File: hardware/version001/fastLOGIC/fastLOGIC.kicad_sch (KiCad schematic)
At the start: 82 parts, among them J1 AVR-ISP-6, J10 0-5V_ANALOG_IN_A, J11 PRES_SENS_BOTTOM, J12 PRES_SENS_TOP, J13 0-5V_ANALOG_IN_B, J14 RELAY_OUT_B, J15 RELAY_OUT_A, J2 USB_B_Micro, J3 DS18B20, J4 12-24V, J5 I2C, J8 12-24V_IN_A, J9 12-24V_IN_B, K1 SANYOU_SRD_Form_C, K2 SANYOU_SRD_Form_C, Q1 MMBT5551L, Q2 MMBT5551L, SW1 SET, SW2 reset, SW3 PLUS, SW4 MINUS, U1 LM78M05_TO252, U2 ATmega328P-A, U3 EL817, U4 EL817, U5 CP2102N-Axx-xQFN28, U6 TM1637, U7 CA56-12SRWA, Y1 Crystal_25MHz

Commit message: hardware chnages minor
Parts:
- removed J2: USB_B_Micro, Connector_USB:USB_Micro-B_Amphenol_10118194_Horizontal, symbol Connector:USB_B_Micro
- added J6: USB_B_Mini, Connector_USB:USB_Mini-B_Tensility_54-00023_Vertical, symbol Connector:USB_B_Mini
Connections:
- net GND: now also J6.5 (GND)
- net at C14.2, C15.2, U5.7 (VREGIN)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: now also J6.1 (VBUS)
- net at U5.5 (D-): now also J6.2 (D-)
- net at U5.4 (D+): now also J6.3 (D+)
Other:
- moved on the sheet: C1, C10, C11, C12, C13, C14, C15, C16, C17, C2, C3, C4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

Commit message: latest pcb
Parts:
- U3, U4: footprint Package_DIP:DIP-4_W7.62mm_SMDSocket_SmallPads -> Package_DIP:DIP-4_W8.89mm_SMDSocket_LongPads
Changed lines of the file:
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@@
       (effects (font (size 1.27 1.27)))
     )
-    (property "Footprint" "Package_DIP:DIP-4_W7.62mm_SMDSocket_SmallPads" (at 54.737 194.691 0)
+    (property "Footprint" "Package_DIP:DIP-4_W8.89mm_SMDSocket_LongPads" (at 54.737 194.691 0)
       (effects (font (size 1.27 1.27) italic) (justify left) hide)
     )
@@
       (effects (font (size 1.27 1.27)))
     )
-    (property "Footprint" "Package_DIP:DIP-4_W7.62mm_SMDSocket_SmallPads" (at 91.821 197.993 0)
+    (property "Footprint" "Package_DIP:DIP-4_W8.89mm_SMDSocket_LongPads" (at 91.821 197.993 0)
       (effects (font (size 1.27 1.27) italic) (justify left) hide)
     )

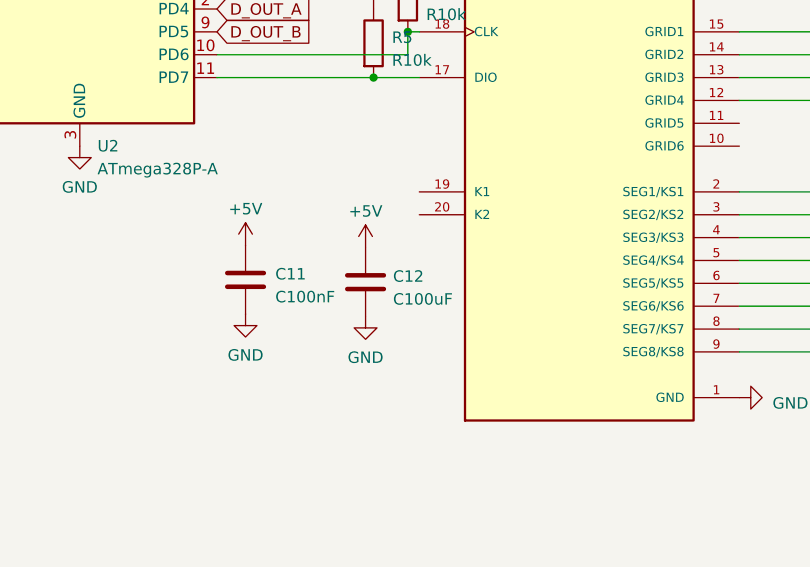
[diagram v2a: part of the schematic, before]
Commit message: minor pcb changes, image
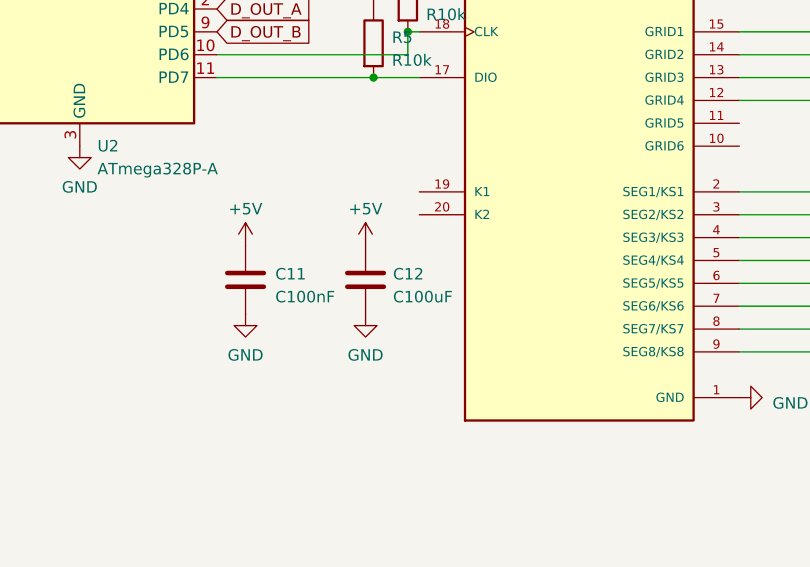
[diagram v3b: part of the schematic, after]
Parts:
- J10, J13, J3: LCSC (none) -> C157928
- J14, J15, J8, J9: LCSC (none) -> C2997510
- J4: LCSC (none) -> C2997509
- J5: LCSC (none) -> C157925
- J6: LCSC (none) -> C6331167
- U7: LCSC (none) -> C38183
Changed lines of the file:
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@@
       (effects (font (size 1.27 1.27)) hide)
     )
+    (property "LCSC" "C157928" (at 229.743 266.827 90)
+      (effects (font (size 1.27 1.27)) hide)
+    )
     (pin "1")
     (pin "2")
@@
       (effects (font (size 1.27 1.27)) hide)
     )
+    (property "LCSC" "C2997509" (at 240.411 266.827 90)
+      (effects (font (size 1.27 1.27)) hide)
+    )
     (pin "1")
     (pin "2")
@@
       (effects (font (size 1.27 1.27)) hide)
     )
+    (property "LCSC" "C2997510" (at 358.013 38.354 90)
+      (effects (font (size 1.27 1.27)) hide)
+    )
     (pin "1")
     (pin "2")
@@
       (effects (font (size 1.27 1.27)) hide)
     )
+    (property "LCSC" "C157928" (at 187.579 266.827 90)
+      (effects (font (size 1.27 1.27)) hide)
+    )
     (pin "1")
     (pin "2")
@@
     )
   )
-  (symbol (lib_id "power:+5V") (at 165.735 117.602 0) (unit 1)
+  (symbol (lib_id "power:+5V") (at 165.735 117.348 0) (unit 1)
     (in_bom yes) (on_board yes) (dnp no) (fields_autoplaced)
-    (property "Reference" "#PWR053" (at 165.735 121.412 0)
+    (property "Reference" "#PWR053" (at 165.735 121.158 0)
       (effects (font (size 1.27 1.27)) hide)
     )
-    (property "Value" "+5V" (at 165.735 113.538 0)
+    (property "Value" "+5V" (at 165.735 113.284 0)
       (effects (font (size 1.27 1.27)))
     )
-    (property "Footprint" "" (at 165.735 117.602 0)
+    (property "Footprint" "" (at 165.735 117.348 0)
       (effects (font (size 1.27 1.27)) hide)
     )
-    (property "Datasheet" "" (at 165.735 117.602 0)
+    (property "Datasheet" "" (at 165.735 117.348 0)
       (effects (font (size 1.27 1.27)) hide)
     )
@@
       (effects (font (size 1.27 1.27)) hide)
     )
+    (property "LCSC" "C157925" (at 257.429 266.827 90)
+      (effects (font (size 1.27 1.27)) hide)
+    )
     (pin "1")
     (pin "2")
@@
     )
   )
-  (symbol (lib_id "Device:C") (at 165.735 121.412 0) (unit 1)
+  (symbol (lib_id "Device:C") (at 165.735 121.158 0) (unit 1)
     (in_bom yes) (on_board yes) (dnp no) (fields_autoplaced)
-    (property "Reference" "C12" (at 168.783 120.777 0)
+    (property "Reference" "C12" (at 168.783 120.523 0)
       (effects (font (size 1.27 1.27)) (justify left))
     )
-    (property "Value" "C100uF" (at 168.783 123.317 0)
+    (property "Value" "C100uF" (at 168.783 123.063 0)
       (effects (font (size 1.27 1.27)) (justify left))
     )
-    (property "Footprint" "Capacitor_SMD:C_1206_3216Metric" (at 166.7002 125.222 0)
+    (property "Footprint" "Capacitor_SMD:C_1206_3216Metric" (at 166.7002 124.968 0)
       (effects (font (size 1.27 1.27)) hide)
     )
-    (property "Datasheet" "~" (at 165.735 121.412 0)
+    (property "Datasheet" "~" (at 165.735 121.158 0)
       (effects (font (size 1.27 1.27)) hide)
     )
-    (property "LCSC" "C15008" (at 165.735 121.412 0)
+    (property "LCSC" "C15008" (at 165.735 121.158 0)
       (effects (font (size 1.27 1.27)) hide)
     )
@@
       (effects (font (size 1.27 1.27)) hide)
     )
+    (property "LCSC" "C2997510" (at 84.201 214.503 90)
+      (effects (font (size 1.27 1.27)) hide)
+    )
     (pin "1")
     (pin "2")
@@
       (effects (font (size 1.27 1.27)) hide)
     )
+    (property "LCSC" "C2997510" (at 47.117 214.249 90)
+      (effects (font (size 1.27 1.27)) hide)
+    )
     (pin "1")
     (pin "2")
@@
       (effects (font (size 1.27 1.27)) hide)
     )
+    (property "LCSC" "C2997510" (at 358.14 87.884 90)
+      (effects (font (size 1.27 1.27)) hide)
+    )
     (pin "1")
     (pin "2")
@@
       (effects (font (size 1.27 1.27)) hide)
     )
+    (property "LCSC" "C38183" (at 244.983 118.999 0)
+      (effects (font (size 1.27 1.27)) hide)
+    )
     (pin "1")
     (pin "10")
@@
     )
   )
-  (symbol (lib_id "power:GND") (at 165.735 125.222 0) (unit 1)
+  (symbol (lib_id "power:GND") (at 165.735 124.968 0) (unit 1)
     (in_bom yes) (on_board yes) (dnp no) (fields_autoplaced)
-    (property "Reference" "#PWR054" (at 165.735 131.572 0)
+    (property "Reference" "#PWR054" (at 165.735 131.318 0)
       (effects (font (size 1.27 1.27)) hide)
     )
-    (property "Value" "GND" (at 165.735 129.794 0)
+    (property "Value" "GND" (at 165.735 129.54 0)
       (effects (font (size 1.27 1.27)))
     )
-    (property "Footprint" "" (at 165.735 125.222 0)
+    (property "Footprint" "" (at 165.735 124.968 0)
       (effects (font (size 1.27 1.27)) hide)
     )
-    (property "Datasheet" "" (at 165.735 125.222 0)
+    (property "Datasheet" "" (at 165.735 124.968 0)
       (effects (font (size 1.27 1.27)) hide)
     )
@@
       (effects (font (size 1.27 1.27)) hide)
     )
+    (property "LCSC" "C6331167" (at 35.814 64.897 0)
+      (effects (font (size 1.27 1.27)) hide)
+    )
     (pin "1")
     (pin "2")
@@
       (effects (font (size 1.27 1.27)) hide)
     )
+    (property "LCSC" "C157928" (at 207.264 266.827 90)
+      (effects (font (size 1.27 1.27)) hide)
+    )
